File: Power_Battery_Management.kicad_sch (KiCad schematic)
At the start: 26 parts, among them J501 S2B-PH-SM4-TB, Q501 NMOS IRLML6344TRPBF SOT-23, Q502 CSD85302L, U501 BQ29737DSER, U502 MCP73831T-2ACI/MC

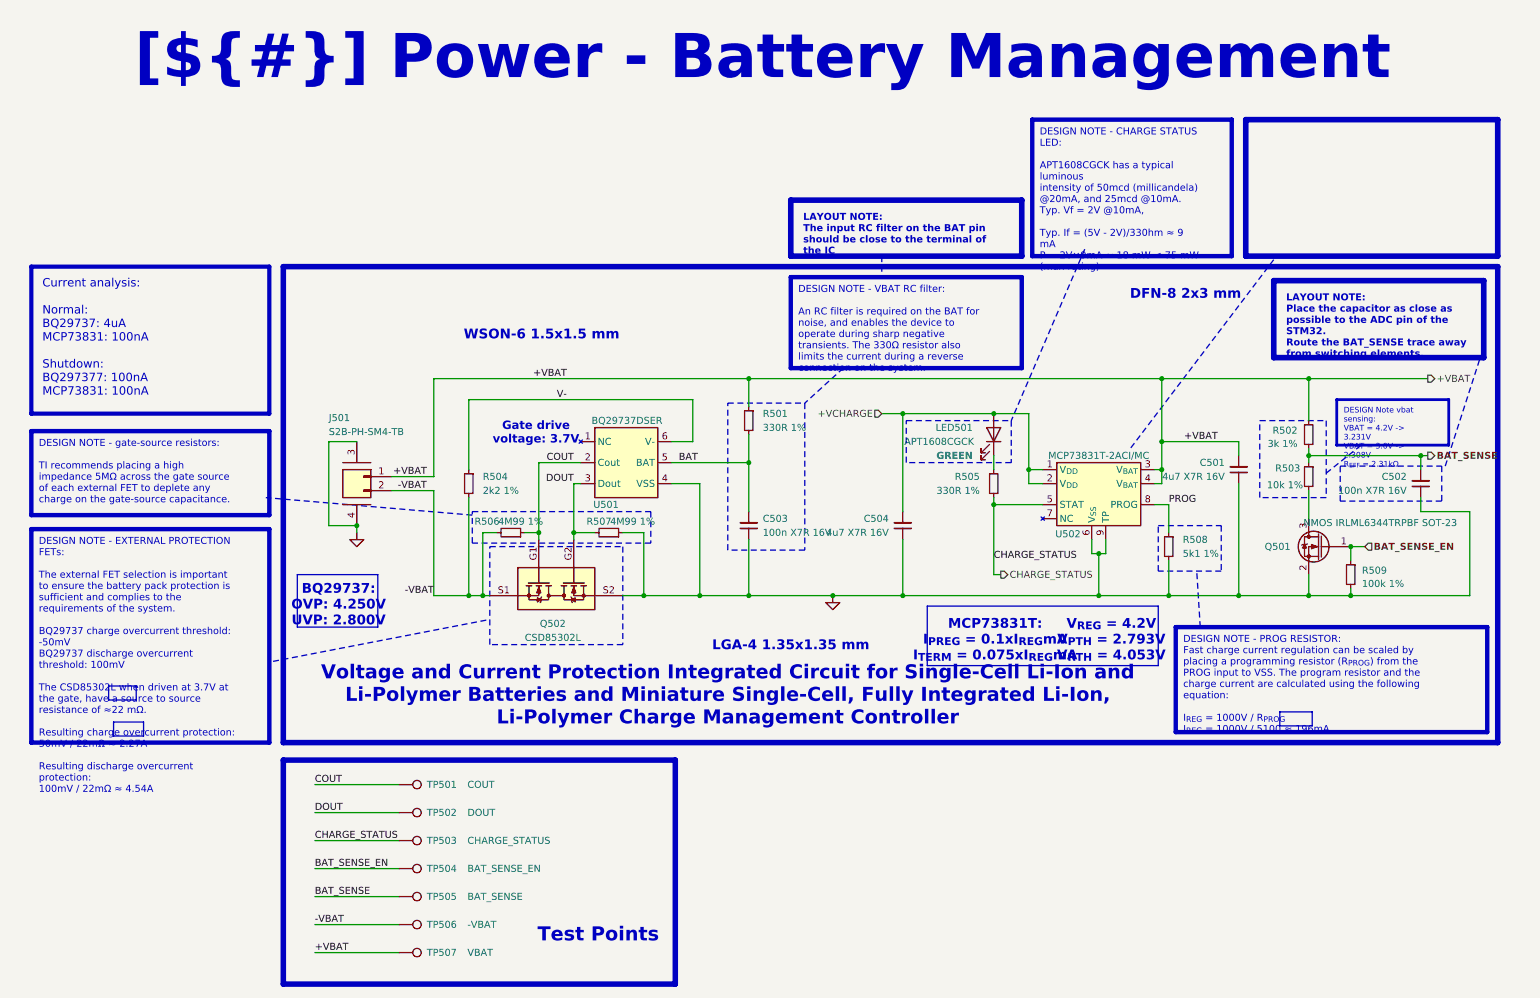
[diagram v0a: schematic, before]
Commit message: Advanced rough layout
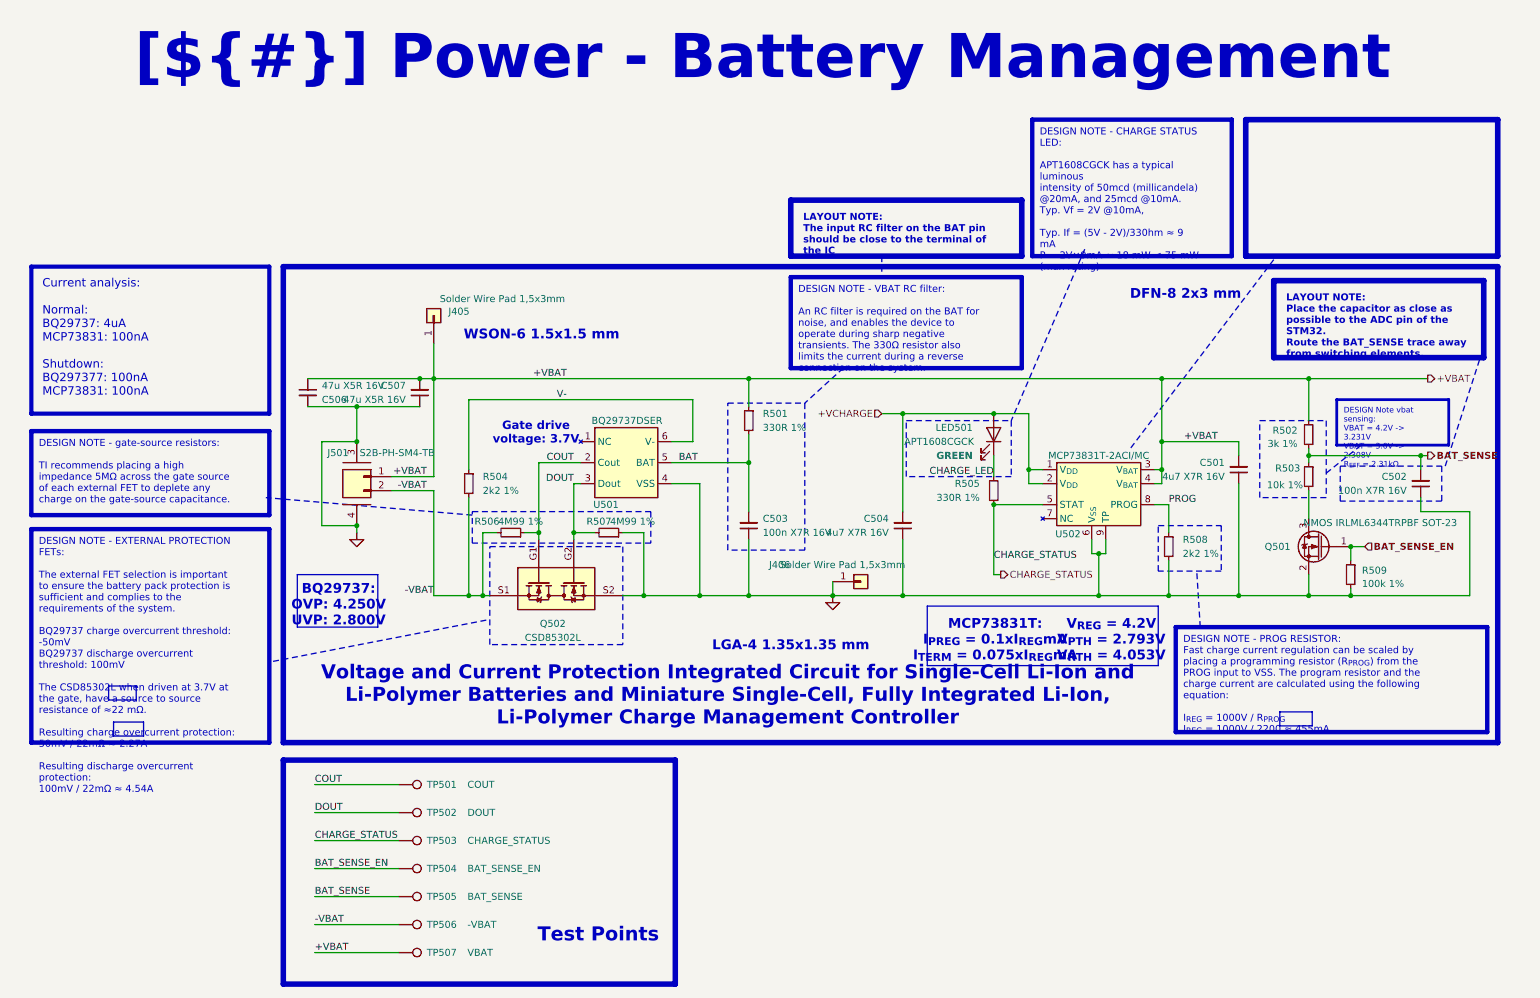
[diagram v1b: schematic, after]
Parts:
- added C506, C507: 47u X5R 16V, Capacitor_SMD:C_1206_3216Metric, symbol Device:C_Small
- added J405, J406: Solder Wire Pad 1,5x3mm, 0_Plume:SolderWirePad_SMD_1,5x3mm, symbol Connector_Generic:Conn_01x01
- R508: value 5k1 1% -> 2k2 1%; Manufacturer Part Number RK73H1ETTP5101F -> RK73H1ETTP2201F; Supplier Part Number 660-RK73H1ETTP5101F -> 660-RK73H1ETTP2201F
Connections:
- net +VBAT: now also C506.1, C507.2, J405.1 (Pin_1)
- net GND: now also C506.2, C507.1, J406.1 (Pin_1)
- net CHARGE_LED: now reaches LED501.1 (K), R505.1
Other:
- moved on the sheet: R505
